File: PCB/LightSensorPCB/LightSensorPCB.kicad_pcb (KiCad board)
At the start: 2 copper layers, 20 x 15 mm, 9 parts, among them J1 POWER/I2C, U1 LTR-329ALS-01

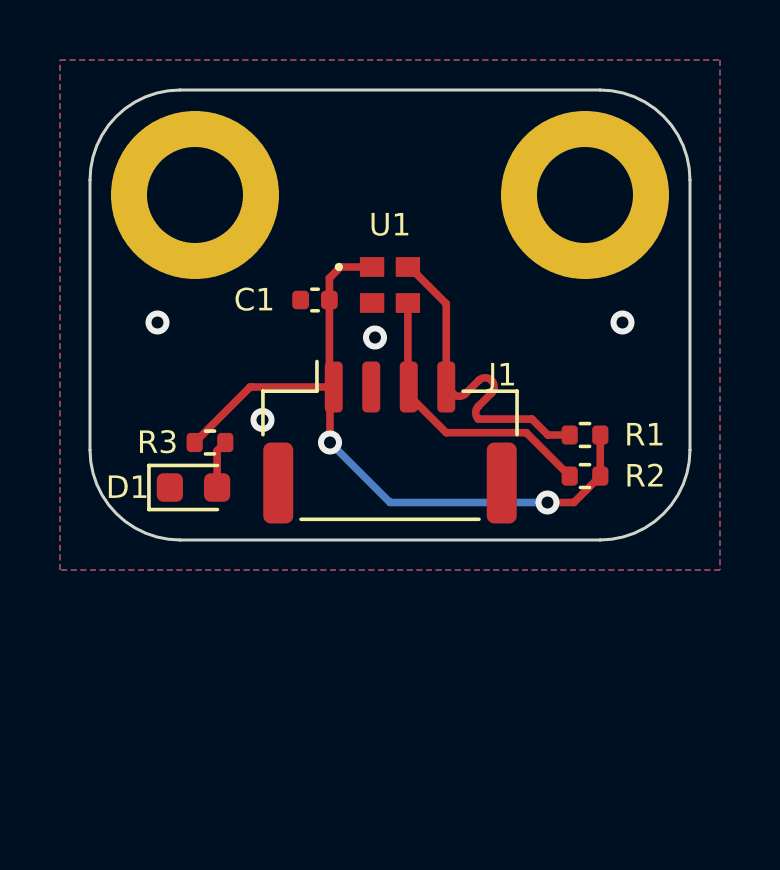
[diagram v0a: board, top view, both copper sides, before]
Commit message: Significant PCB progress
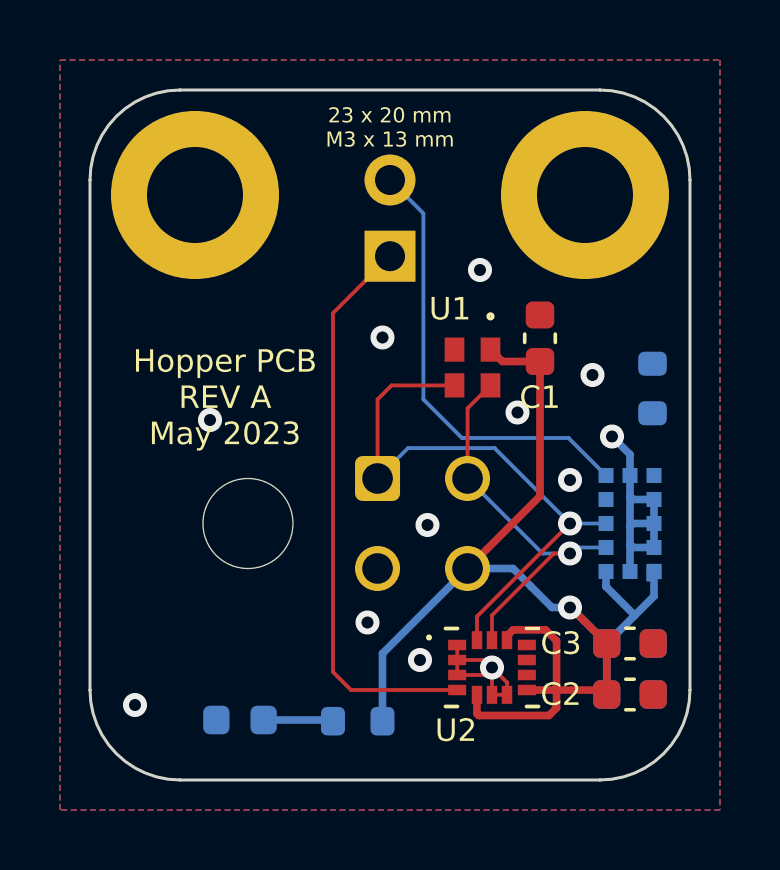
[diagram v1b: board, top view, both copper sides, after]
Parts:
- removed R1, R2: 10kOhm 1% 0402, Resistor_SMD:R_0402_1005Metric
- added C2: 0.1 uF 50V X7R 0603, Capacitor_SMD:C_0603_1608Metric, F.Cu at (118.0, 120.2)
- added C3: 0.1 uF 50V X7R 0603, Capacitor_SMD:C_0603_1608Metric, F.Cu at (118.0, 118.5)
- added C4: 4.7 uF 6.3V X5R 0603, Capacitor_SMD:C_0603_1608Metric, B.Cu at (118.0, 120.2)
- added C5: 0.1 uF 50V X7R 0603, Capacitor_SMD:C_0603_1608Metric, B.Cu at (118.0, 118.5)
- added R4: 10kOhm 1% 0603, Resistor_SMD:R_0603_1608Metric, B.Cu at (118.8, 110.0)
- added TP1: TestPoint_2Pole, Connector_PinHeader_2.54mm:PinHeader_1x02_P2.54mm_Vertical, B.Cu at (110.0, 105.5)
- added U2: LSM6DSMTR, Customs:PQFN50P300X250X86-14N, F.Cu at (113.4, 119.2)
- added U3: VL53L3CXV0DH/1, Customs:XDCR_VL53L3CXV0DH_1, B.Cu at (118.0, 114.5)
- C1: value 1 uF 6.3V X7R 0402 -> 1 uF 25V X5R 0603; footprint Capacitor_SMD:C_0402_1005Metric -> Capacitor_SMD:C_0603_1608Metric
- D1: value RED 1.8V 2mA -> RED 1.8V 2mA 0603; moved to B.Cu
- J1: footprint Connector_JST:JST_GH_SM04B-GHS-TB_1x04-1MP_P1.25mm_Horizontal -> Connector_Molex:Molex_Micro-Fit_3.0_43045-0400_2x02_P3.00mm_Horizontal; moved to B.Cu
- R3: value 750Ohm 1% 0402 -> 750Ohm 1% 0603; footprint Resistor_SMD:R_0402_1005Metric -> Resistor_SMD:R_0603_1608Metric; moved to B.Cu
- moved H1 13.0 mm to (103.5, 103.5)
- moved H2 13.0 mm to (116.5, 103.5)
- moved R3 10.5 mm to (108.9, 121.0), turned to 0 degrees
- moved D1 7.90 mm to (105.0, 121.0)
- moved C1 7.61 mm to (115.0, 108.3), turned to 90 degrees
- moved U1 3.89 mm to (112.8, 109.2), turned to -90 degrees
- moved J1 1.27 mm to (109.6, 113.0), turned to -90 degrees
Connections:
- J1 pad 1: +3.3V -> /SDA
- J1 pad 3: /SDA -> /SCL
- J1 pad 4: /SCL -> +3.3V
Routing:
- net /GPIO_LSM: track 0.00 -> 19.0 mm
- net +3.3V: track 24.1 -> 42.1 mm, vias 2 -> 1
- net GND: track 0.00 -> 14.9 mm, vias 4 -> 12
- net /GPIO_VL5: track 0.00 -> 14.9 mm
- net /SDA: track 9.57 -> 19.9 mm, vias 0 -> 1
- net /SCL: track 11.2 -> 13.4 mm, vias 0 -> 1
- net Net-(D1-Pad2): track 1.61 -> 2.33 mm
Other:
- board size 20 x 15 mm -> 20 x 23 mm
- board text added: "+3.3V"
- board text added: "23 x 20 mm M3 x 13 mm"
- board text added: "Hopper PCB REV A May 2023"
- board text added: "INT1"
- board text added: "VL51"
